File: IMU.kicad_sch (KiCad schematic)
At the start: 7 parts, among them J3 5033981892, U1 ICM-42688-P

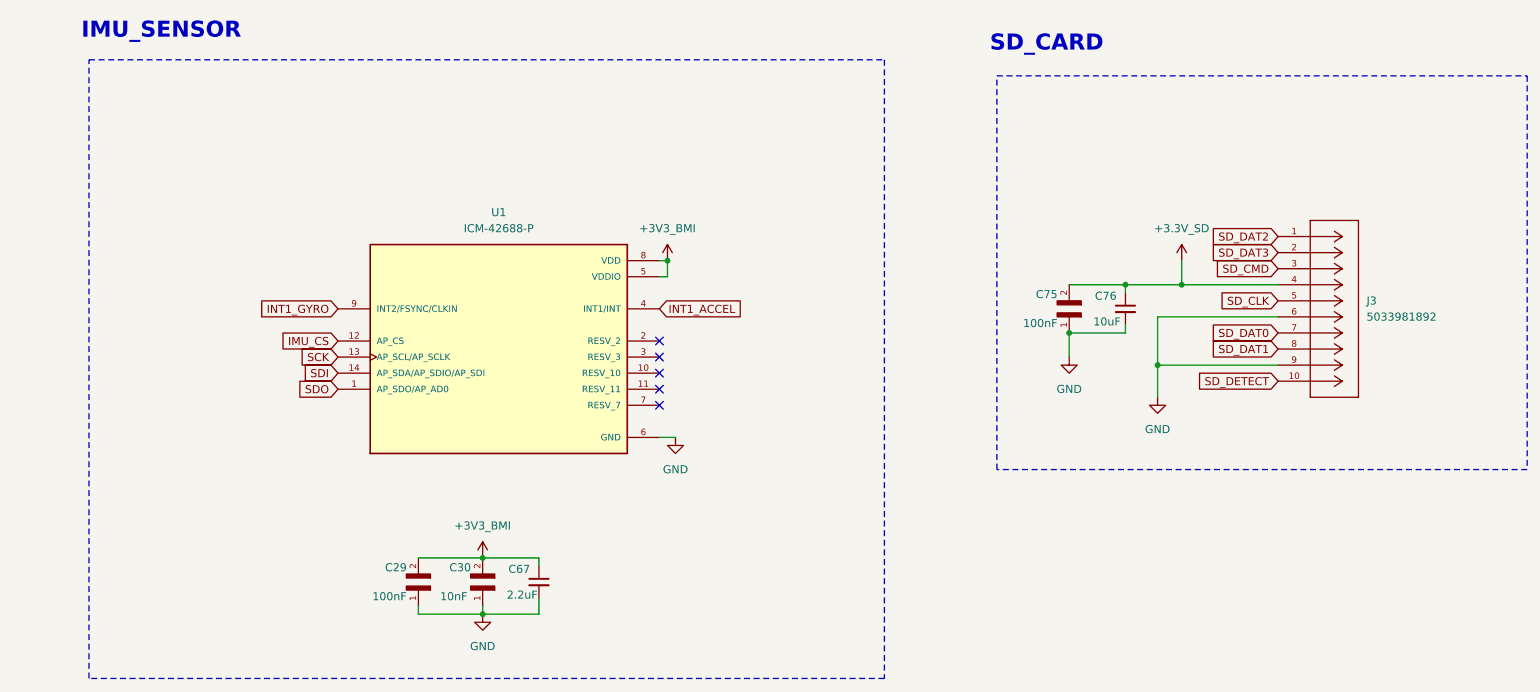
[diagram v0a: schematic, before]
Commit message: new
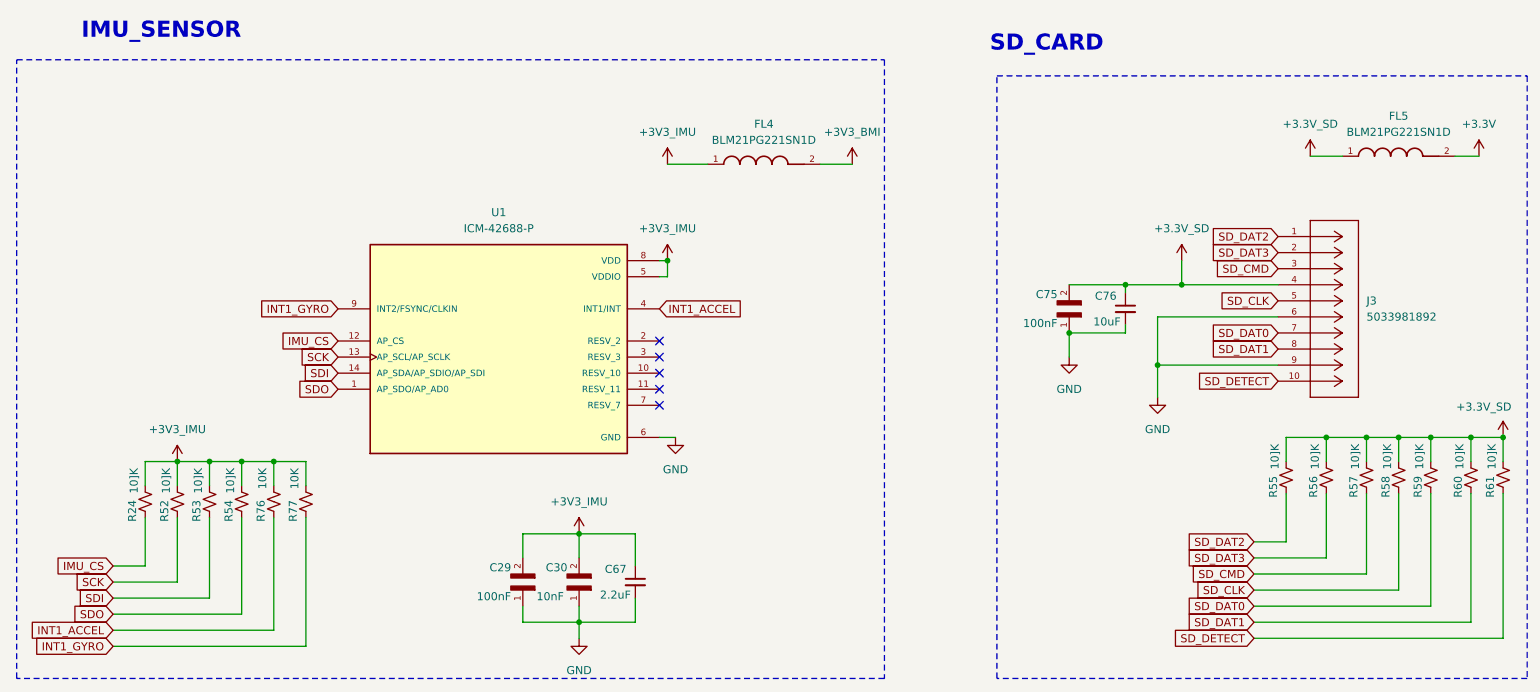
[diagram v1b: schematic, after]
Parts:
- added FL4, FL5: BLM21PG221SN1D, BLM21PG221SN1D:BEADC2012X105N, symbol BLM21PG221SN1D:BLM21PG221SN1D
- added R24, R52, R53, R54, R55, R56, R57, R58, R59, R60, R61: 10]K, Resistor_SMD:R_0805_2012Metric, symbol Device:R_Small_US
- added R76, R77: 10K, Resistor_SMD:R_0805_2012Metric, symbol Device:R_Small_US
- J3: footprint GNSS_Library:CONN_503398-1892_MOL -> GNSS:CONN_503398-1892_MOL
- U1: footprint ICM-42688-P:PQFN50P300X250X97-14N -> GNSS:PQFN50P300X250X97-14N
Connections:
- net +3.3V_SD: now also FL5.1, R55.2, R56.2, R57.2, R58.2, R59.2, R60.2, R61.2
- net +3V3_BMI: now also FL4.2; no longer C29.2, C30.2, C67.1, U1.5 (VDDIO), U1.8 (VDD)
- net IMU_CS: now also R24.1
- net INT1_ACCEL: now also R76.1
- net INT1_GYRO: now also R77.1
- net SCK: now also R52.1
- net SDI: now also R53.1
- net SDO: now also R54.1
- net SD_CLK: now also R58.1
- net SD_CMD: now also R57.1
- net SD_DAT0: now also R59.1
- net SD_DAT1: now also R60.1
- net SD_DAT2: now also R55.1
- net SD_DAT3: now also R56.1
- net SD_DETECT: now also R61.1
- new net +3.3V: FL5.2
- new net +3V3_IMU: C29.2, C30.2, C67.1, FL4.1, R24.2, R52.2, R53.2, R54.2, R76.2, R77.2, U1.5 (VDDIO), U1.8 (VDD)
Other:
- moved on the sheet: C29, C30, C67
